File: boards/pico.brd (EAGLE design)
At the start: 93.3 x 53.3 mm, 54 parts, among them IC3 ULN2803A, IC4 ULN2803A, J1 RS232, U2 ATMEGA32U4-XUAU, X1 16MHz, X2 MINI-USB-UX60-MB-5ST

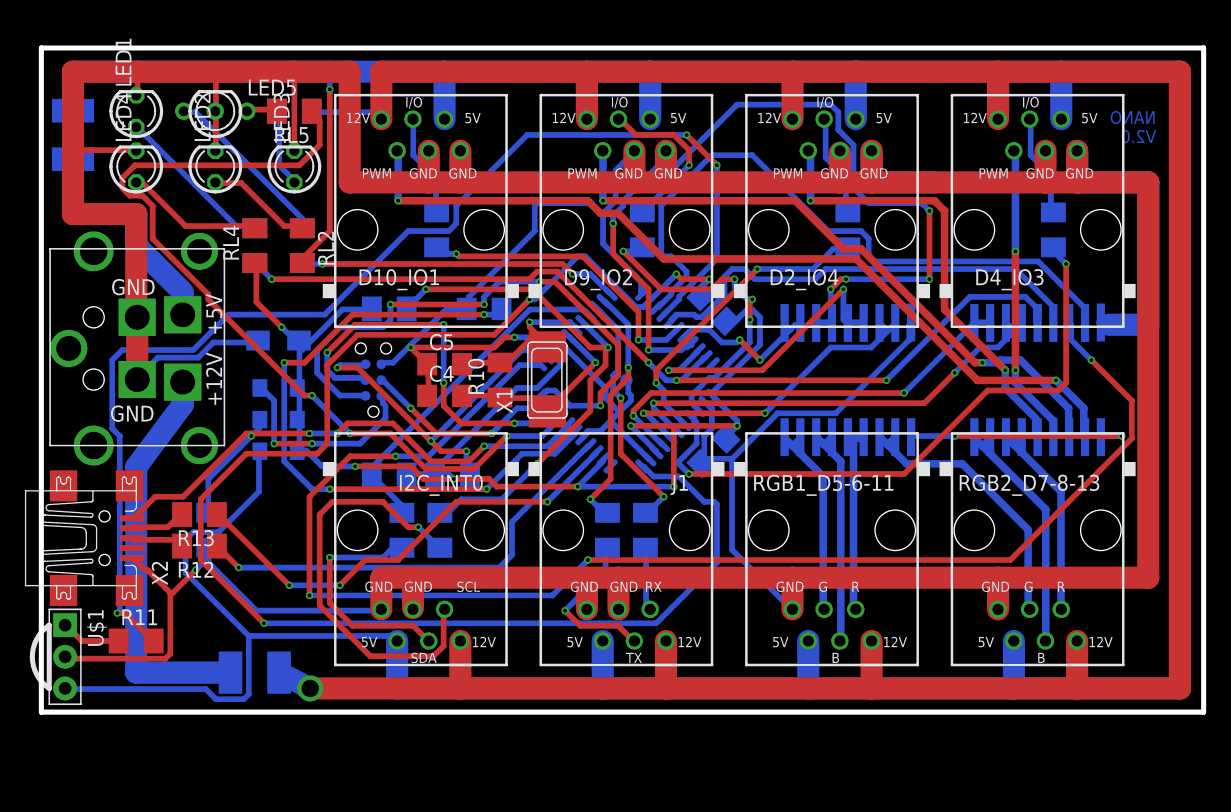
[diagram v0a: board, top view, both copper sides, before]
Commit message: put all the downloaded files into directories
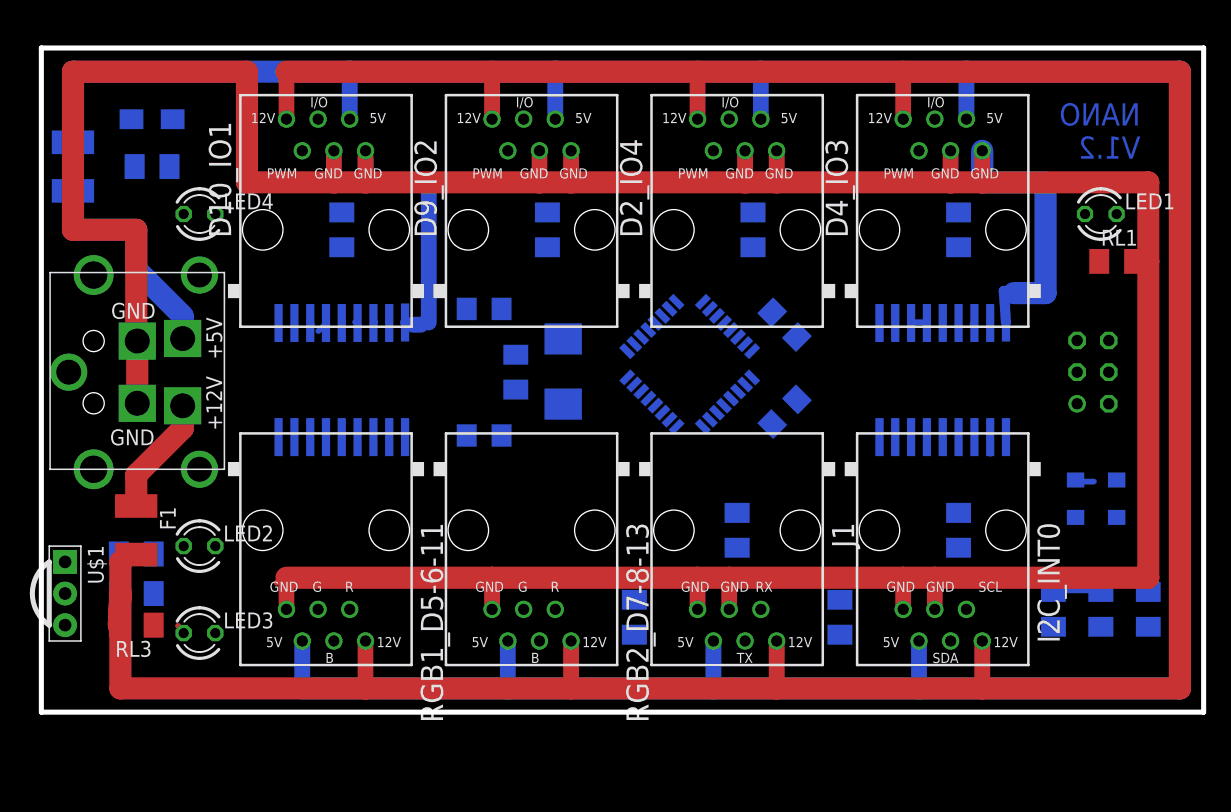
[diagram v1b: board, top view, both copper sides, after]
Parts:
- removed C6: 1uF, resistor:C1206
- removed C7: 10uF, resistor:C1206
- removed D3: 1N581D1206, lpatiny:LED-1206
- removed LED5: BICOLOR-LED, lpatiny:BICOLOR-3MM
- removed R12, R13: 22, resistor:M1206
- removed RL5, RL6: 1K, resistor:M1206
- removed U2: ATMEGA32U4-XUAU, SmartPrj:TQFP44-PAD
- removed X2: MINI-USB-UX60-MB-5ST, con-hirose:UX60-MB-5ST
- added IC1: MEGA8-AI, atmel:TQFP32-08
- CON1: device lpatiny:TC2030-MCP-NL -> lpatiny:TINYISP
- LED2: value 5V -> (none)
- LED3: value 12V -> (none)
- LED4: value 5V uC -> (none)
- moved LED1 77.9 mm to (85.1, 39.4), turned to 0 degrees
- moved RL1 69.2 mm to (86.4, 35.6), flipped to the top, turned to 0 degrees
- moved D1 67.9 mm to (86.4, 16.5), turned to 270 degrees
- moved D2 64.1 mm to (83.1, 16.5), turned to 270 degrees
- moved R7 62.0 mm to (85.1, 7.62), turned to 270 degrees
- moved CON1 57.9 mm to (84.5, 26.7)
- moved R1 56.9 mm to (88.9, 7.62), turned to 270 degrees
- moved R6 49.7 mm to (81.3, 7.62)
- moved R2 44.7 mm to (73.7, 14.0), turned to 270 degrees
- moved RL3 43.2 mm to (7.62, 6.35), flipped to the top
- moved I2C_INT0 41.9 mm to (72.4, 14.0)
- moved RGB2_D7-8-13 40.6 mm to (39.4, 14.0)
- moved IC4 40.6 mm to (24.1, 26.0)
- moved RGB1_D5-6-11 40.6 mm to (22.9, 14.0)
- moved LED3 38.2 mm to (12.7, 5.71), turned to 0 degrees
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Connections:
- removed net D+: R12.2, X2.3
- removed net D-: R13.2, X2.2
- removed net D11: IC3.7, U2.12
- removed net D12: R11.2, U2.26
- removed net D13: IC3.5, RL1.1, U2.32
- removed net D18: R4.2, U2.36
- removed net D19: R1B.2, U2.37
- removed net D20: R0.2, U2.38
- removed net D21: IC3.3, IC3.4, U2.39
- removed net D22: IC4.7, IC4.8, U2.40
- removed net D23: IC3.1, IC3.2, U2.41
- removed net HWB: U2.33
- removed net N$10: C1.2, U2.24, U2.44
- removed net N$11: LED5.3, RL5.2
- removed net N$12: LED5.1, RL6.2
- removed net N$13: IC3.15, IC3.16, RGB2_D7-8-13.R
- removed net RD+: R12.1, U2.4
- removed net RD-: R13.1, U2.3
- removed net RXLED: RL5.1, U2.8
- removed net TXLED: RL6.1, U2.22
- removed net VUSB: C7.2, D3.A, U2.7, X2.1
- new net A0: IC1.23, R0.2
- new net A1: IC1.24, R1B.2
- new net A2: IC1.25, R4.2
- new net A3: IC1.26, R9.2
- new net A6: IC1.19
- new net A7: IC1.22
- new net D2: IC1.32, IC3.5
- new net D3: IC1.1, R11.2
- new net N$5: IC4.11, IC4.12, RGB2_D7-8-13.R
- net 5V: now also IC1.18, IC1.4, IC1.6; no longer D3.C, U2.14, U2.2, U2.34, U2.42
- net D10: now also IC1.14, IC3.8; no longer IC4.3, IC4.4, U2.30
- net D14: now also IC1.7; no longer U2.16
- net D15: now also IC1.8; no longer U2.17
- net D4: now also IC1.2, IC3.6; no longer IC3.8, U2.25
- net D5: now also IC1.9, IC4.1, IC4.2; no longer IC4.5, IC4.6, U2.31
- net D6: now also IC1.10, IC4.3, IC4.4; no longer IC3.6, U2.27
- net D7: now also IC1.11, IC4.7, IC4.8; no longer U2.1
- net D8: now also IC1.12, IC3.1, IC3.2; no longer R9.2, U2.28
- net D9: now also IC1.13, IC3.7; no longer IC4.1, IC4.2, U2.29
- net GND: now also IC1.21, IC1.3, IC1.5, RL1.2; no longer C6.2, C7.1, LED1.K, LED5.2, U2.15, U2.23, U2.35, U2.43, U2.5, U2.P$1, X2.5
- net ISP+5V: now also CON1.VCC; no longer CON1.5V
- net MISO: now also IC1.16; no longer U2.11
- net MOSI: now also IC1.15, IC4.5, IC4.6; no longer U2.10
- net N$1: now also IC4.13, IC4.14; no longer IC4.17, IC4.18
- net N$3: now also LED1.K, RL1.1; no longer LED1.A, RL1.2
- net N$4: now also C1.2, IC1.20; no longer C6.1, U2.6
- net N$57: now also IC3.15, IC3.16; no longer IC4.11, IC4.12
- net N$68: now also IC4.17, IC4.18; no longer IC4.13, IC4.14
- net RESET: now also IC1.29; no longer U2.13
- net RX: now also IC1.30; no longer U2.20
- net SCK: now also IC1.17, IC3.3, IC3.4, LED1.A; no longer U2.9
- net SCL: now also IC1.28; no longer U2.18
- net SDA: now also IC1.27; no longer U2.19
- net TX: now also IC1.31; no longer U2.21
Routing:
- net GND: track 475.7 -> 311.6 mm, vias 3 -> 0
- net N$10: track 119.6 -> 0.00 mm, vias 4 -> 0
- net D11: track 113.5 -> 0.00 mm, vias 4 -> 0
- net 5V: track 112.1 -> 0.23 mm, vias 7 -> 0
- net D12: track 96.2 -> 0.00 mm, vias 3 -> 0
- net D13: track 74.7 -> 0.00 mm, vias 4 -> 0
- net RXLED: track 69.7 -> 0.00 mm, vias 3 -> 0
- net D10: track 69.3 -> 0.00 mm, vias 6 -> 0
- net N$51: track 68.4 -> 1.33 mm, vias 2 -> 0
- net +5V: track 303.8 -> 246.8 mm, vias 1 -> 0
- net D4: track 54.6 -> 0.17 mm
- net N$4: track 53.5 -> 0.00 mm, vias 4 -> 0
- net N$22: track 50.8 -> 0.00 mm, vias 2 -> 0
- net D19: track 50.3 -> 0.00 mm, vias 2 -> 0
- net VUSB: track 50.2 -> 0.00 mm, vias 4 -> 0
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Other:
- board text added: "NANO V1.2"
- board text removed: "NANO V2.0"
